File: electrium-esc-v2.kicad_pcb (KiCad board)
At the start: 2 copper layers, 75.4 x 42 mm, 76 parts, among them IC1 LMR36510FADDAR, J1 CAN, J2 USB_B_Micro, J3 GPIO, J4 Conn_01x02, J5 Debugger Pins, J6 Conn_01x03_Pin, Q1 IRF3205, Q2 IRF3205, Q3 IRF3205, Q4 IRF3205, Q5 IRF3205, Q6 IRF3205, U1 NCP1117-3.3_SOT223, U2 W25Q128JVS, U3 RP2040, U4 DRV8323HRTAR, U5 NRF24L01_Breakout, U6 SN65HVD233, Y1 ABLS-12.000MHZ-B4-T

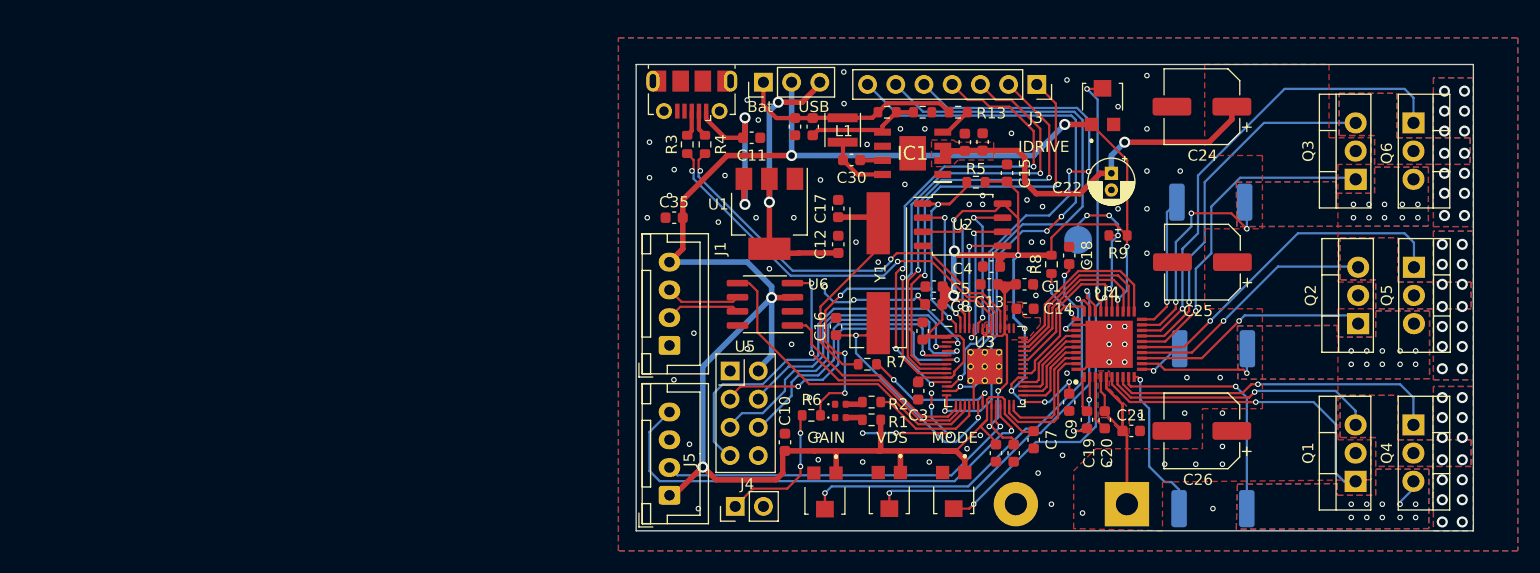
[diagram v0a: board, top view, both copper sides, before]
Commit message: minor improvements
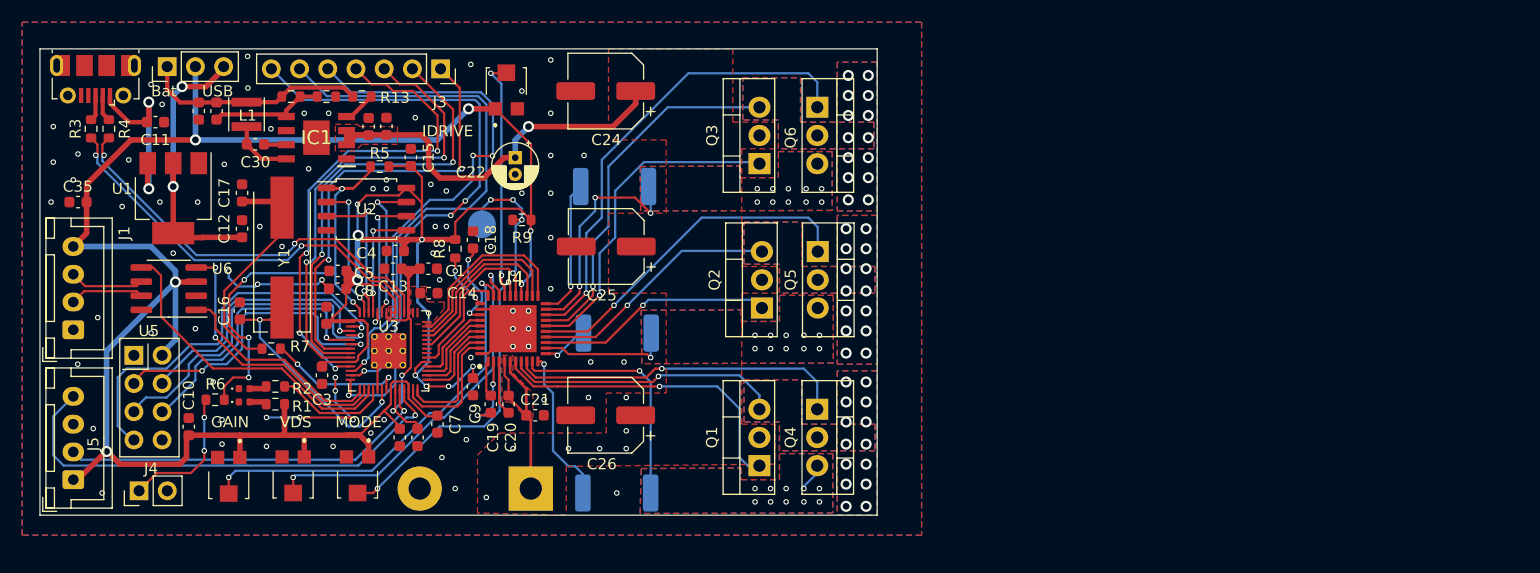
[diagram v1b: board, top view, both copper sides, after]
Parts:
- moved C35 53.7 mm to (124.7, 87.6)
- moved C1 53.7 mm to (156.3, 93.6)
- moved C10 53.7 mm to (134.7, 107.8)
- moved C11 53.7 mm to (131.7, 80.4)
- moved C12 53.7 mm to (139.5, 90.0)
- moved C13 53.7 mm to (153.1, 93.6)
- moved C14 53.7 mm to (156.3, 95.8)
- moved C15 53.7 mm to (154.7, 83.6)
- moved C16 53.7 mm to (139.3, 97.4)
- moved C17 53.7 mm to (139.5, 86.8)
- moved C18 53.7 mm to (160.3, 91.0)
- moved C19 53.7 mm to (161.9, 105.8)
- moved C2 53.7 mm to (155.3, 108.8)
- moved C20 53.7 mm to (163.5, 105.8)
- moved C21 53.7 mm to (165.9, 106.8)
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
